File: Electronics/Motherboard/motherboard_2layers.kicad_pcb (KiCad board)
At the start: 2 copper layers, 113.4 x 56 mm, 56 parts, among them J2 Conn_02x10_Odd_Even, M1 AO3400A, M2 AO3400A, M3 AO3400A, U1 AMS1117-3.3, U6 LM2576HVS-5, U8 STM32F405RGTx

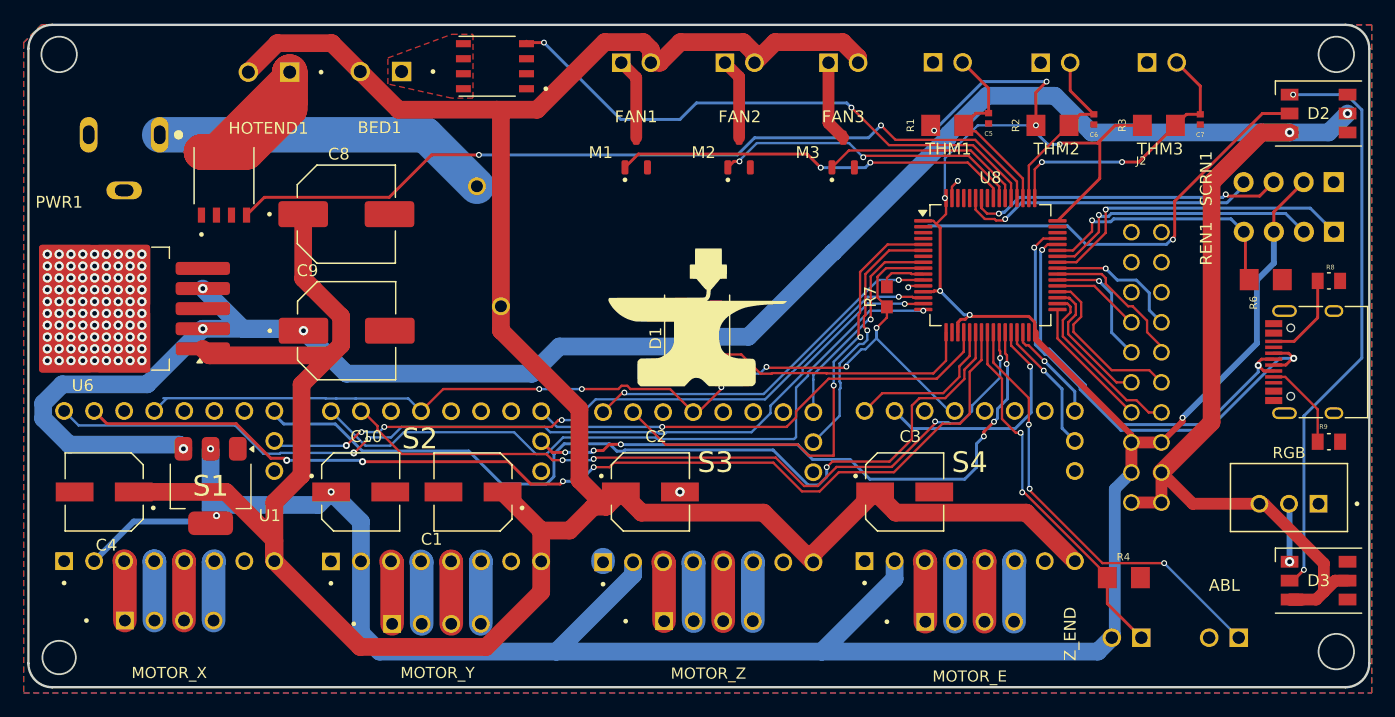
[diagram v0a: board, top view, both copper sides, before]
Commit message: more clean up neneds to be done
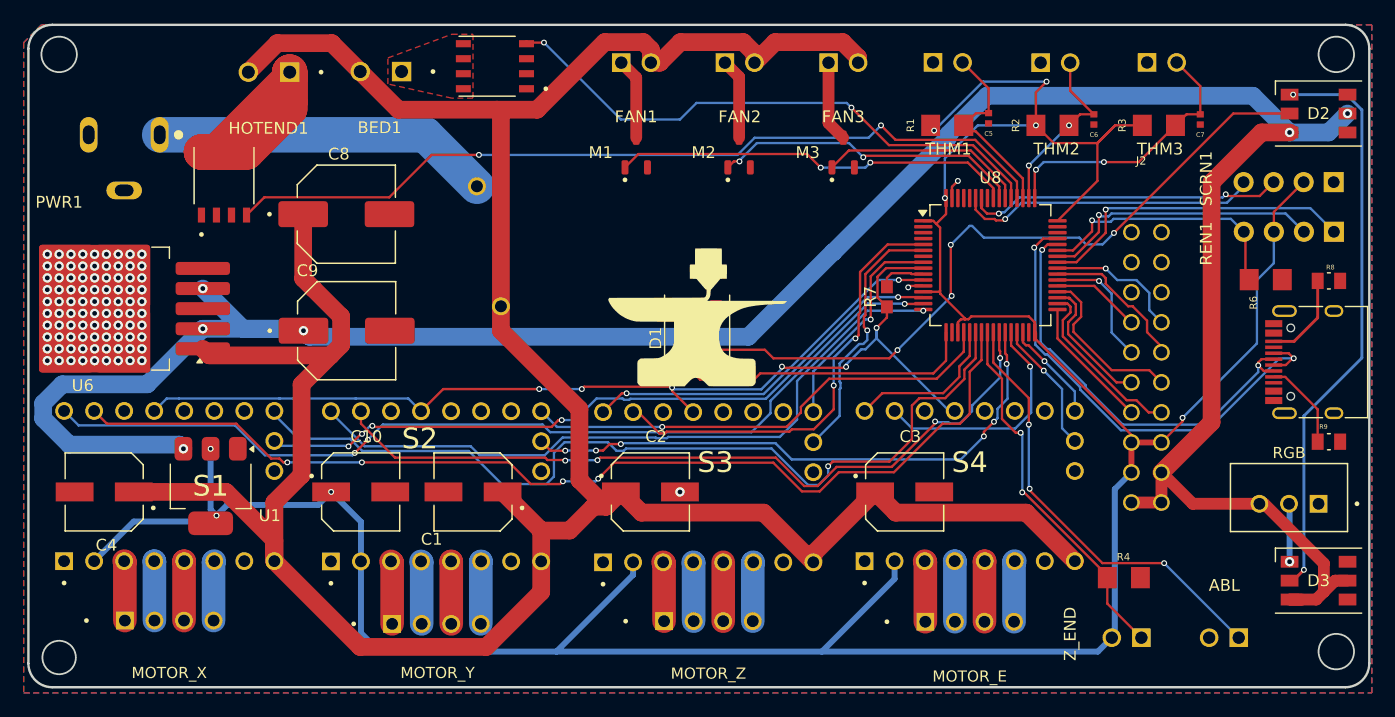
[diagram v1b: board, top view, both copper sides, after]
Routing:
- net Net-(D1-DOUT): track 37.7 -> 65.5 mm, vias 1 -> 4
- net STEP_M2: track 41.5 -> 37.5 mm
- net +5V: track 221.6 -> 218.9 mm
- net DIAG_M3: track 51.8 -> 49.2 mm
- net DIR_M3: track 60.3 -> 58.7 mm
- net UART_RX: track 87.1 -> 88.4 mm
- net +3V3: track 257.3 -> 256.7 mm, vias 11 -> 8
- net T1: vias 0 -> 2
